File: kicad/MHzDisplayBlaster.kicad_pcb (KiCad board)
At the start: 2 copper layers, 50 x 39 mm, 7 parts, among them J1 Conn_02x15 DigitRHS, J2 Conn_02x15 DigitLHS, J3 Conn_01x03_Pin, U1 DC56-11GWA, U2 74LS04

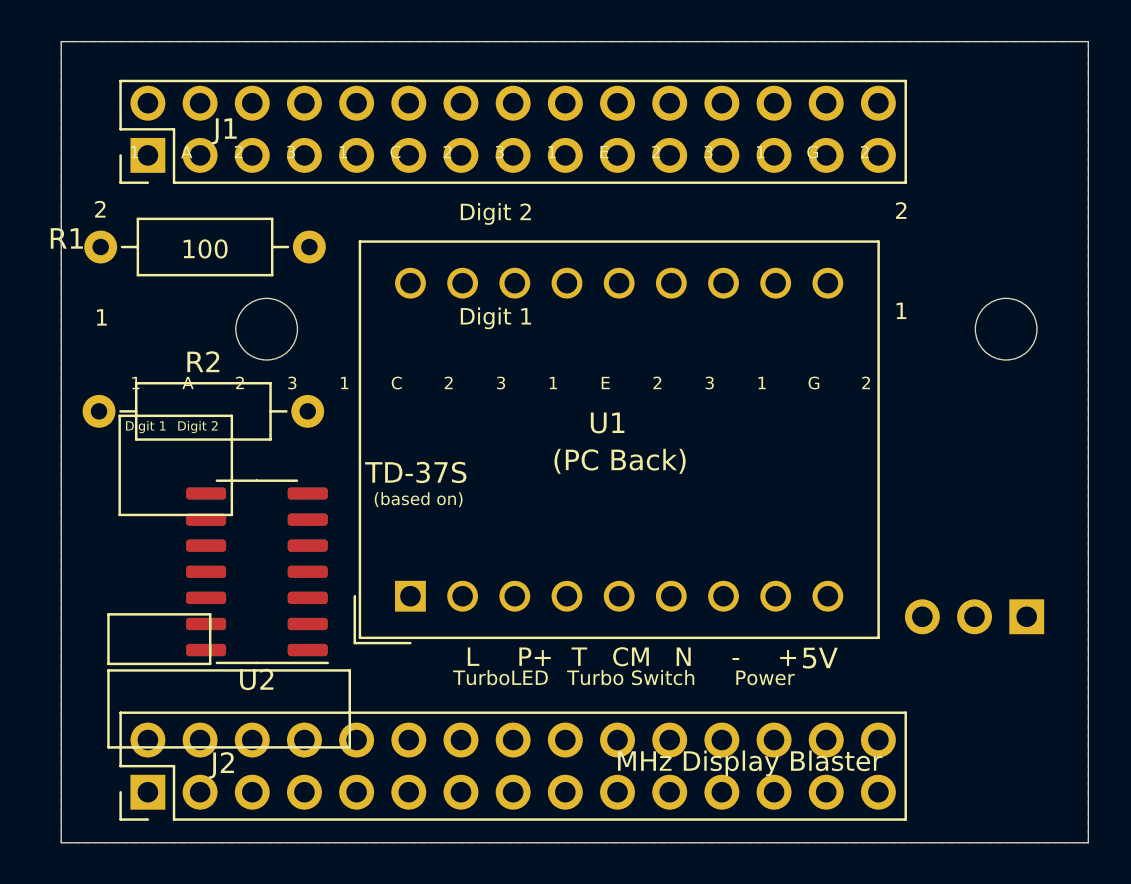
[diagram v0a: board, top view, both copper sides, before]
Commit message: Cleanup and Routing
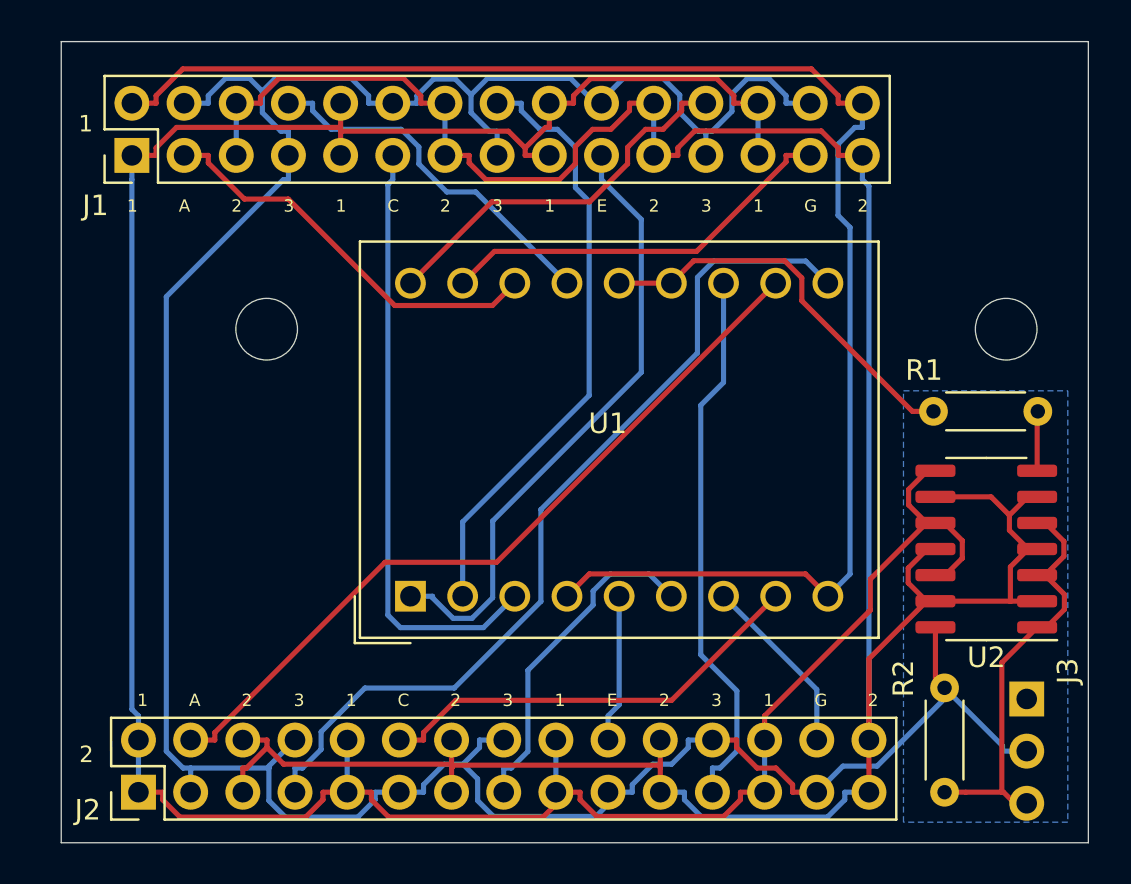
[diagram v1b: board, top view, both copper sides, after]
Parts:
- R1, R2: footprint Resistor_THT:R_Axial_DIN0207_L6.3mm_D2.5mm_P10.16mm_Horizontal -> Resistor_THT:R_Axial_DIN0204_L3.6mm_D1.6mm_P5.08mm_Horizontal
- moved R1 46.3 mm to (147.5, 58.0), turned to 180 degrees
- moved R2 43.3 mm to (143.0, 71.5), turned to -90 degrees
- moved U2 35.5 mm to (145.0, 64.7)
- moved J1 31.0 mm to (103.4, 45.5)
- moved J2 31.0 mm to (103.8, 76.5)
- moved J3 4.00 mm to (147.0, 72.0), turned to 180 degrees
- renumbered J2 to J1, J1 to J2
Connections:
- J3 pad 1: Turbo -> GND
- J3 pad 3: GND -> Turbo
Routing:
- net 2: track 0.00 -> 143.5 mm
- net 3: track 0.00 -> 143.2 mm
- net 1: track 0.00 -> 137.2 mm
- net DP: track 0.00 -> 76.4 mm
- net DIG2_B: track 0.00 -> 43.1 mm
- net DIG2_A: track 0.00 -> 37.9 mm
- net DIG1_E: track 0.00 -> 30.2 mm
- net DIG1_D: track 0.00 -> 29.6 mm
- net DIG1_C: track 0.00 -> 29.5 mm
- net DIG2_F: track 0.00 -> 26.7 mm
- net DIG2_C: track 0.00 -> 21.4 mm
- net Turbo: track 0.00 -> 20.8 mm
- net DIG1_A: track 0.00 -> 19.8 mm
- net DIG1_G: track 0.00 -> 19.7 mm
- net DIG1_CC: track 0.00 -> 19.4 mm
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- added copper zone on B.Cu, net GND
- removed copper zone on F.Cu, net 3
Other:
- board text added: "+5"
- board text added: "Gnd"
- board text added: "Trbo"
- board text removed: "(PC Back)"
- board text removed: "(PC Front)"
- board text removed: "(based on)"
- board text removed: "+"
- board text removed: "-"
- board text removed: "10"
- board text removed: "18"
- board text removed: "1: Turbo OFF 2: Turbo ON 3: Always ON"
- board text removed: "5V"
- board text removed: "7-Segment Display Common Cathode 0.56""
- board text removed: "B"
- board text removed: "CM"
- board text removed: "D"
- board text removed: "DP"
- board text removed: "Digit 1"
- board text removed: "Digit 2"
- board text removed: "F"
- board text removed: "L"
- board text removed: "N"
- board text removed: "P"
- board text removed: "Power"
- board text removed: "Scrap Computing"
- board text removed: "T"
- board text removed: "TD-37S"
- board text removed: "Turbo Switch"
- board text removed: "TurboLED"
- board text removed: "by Scrap Computing"
- board text removed: "rev.0.2"
